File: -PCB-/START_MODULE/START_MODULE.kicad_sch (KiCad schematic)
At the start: 8 parts, among them J1 Conn_01x03_Pin, J2 Conn_01x04_Pin, U1 ATtiny85-20S, U2 TSOP382xx

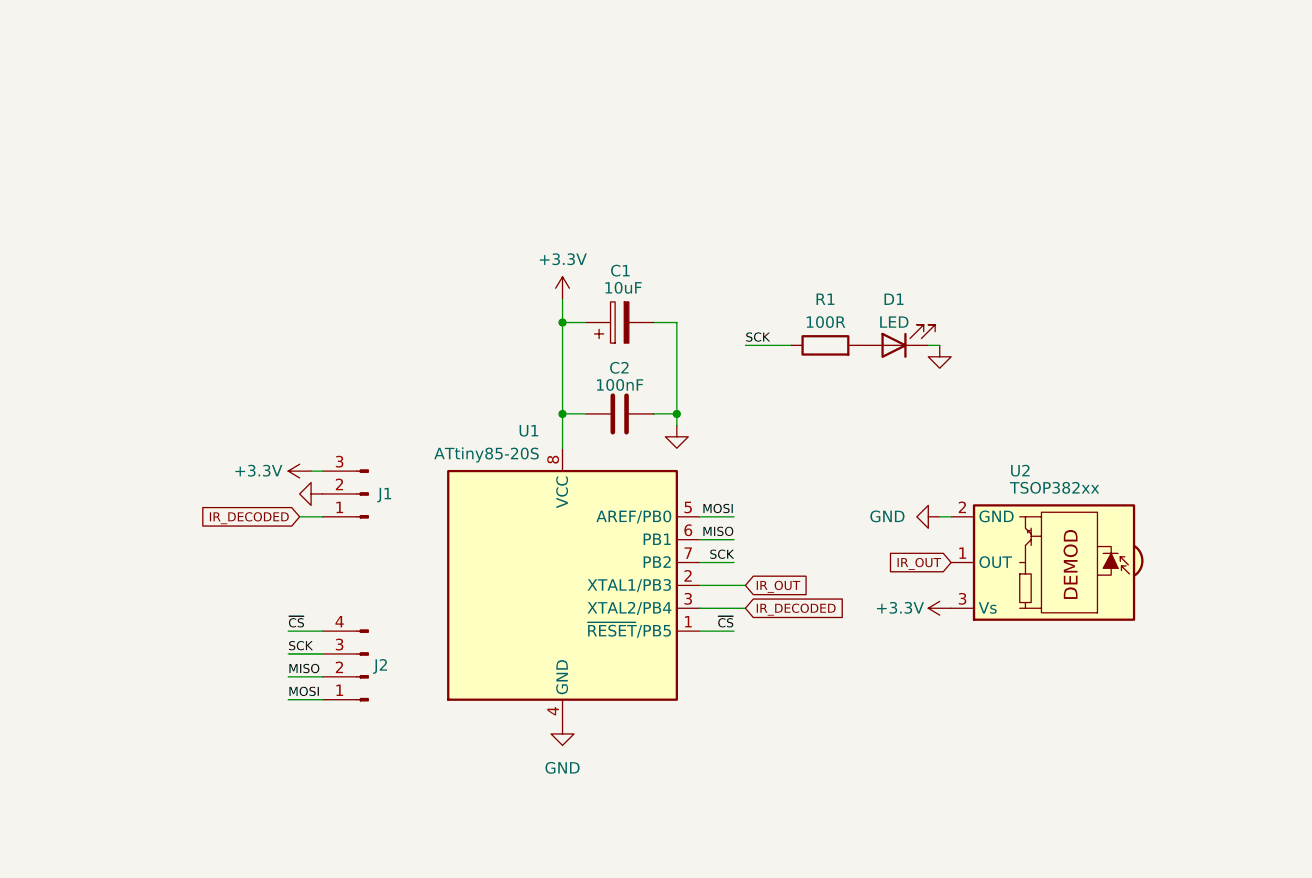
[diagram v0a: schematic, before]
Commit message: IR_module update
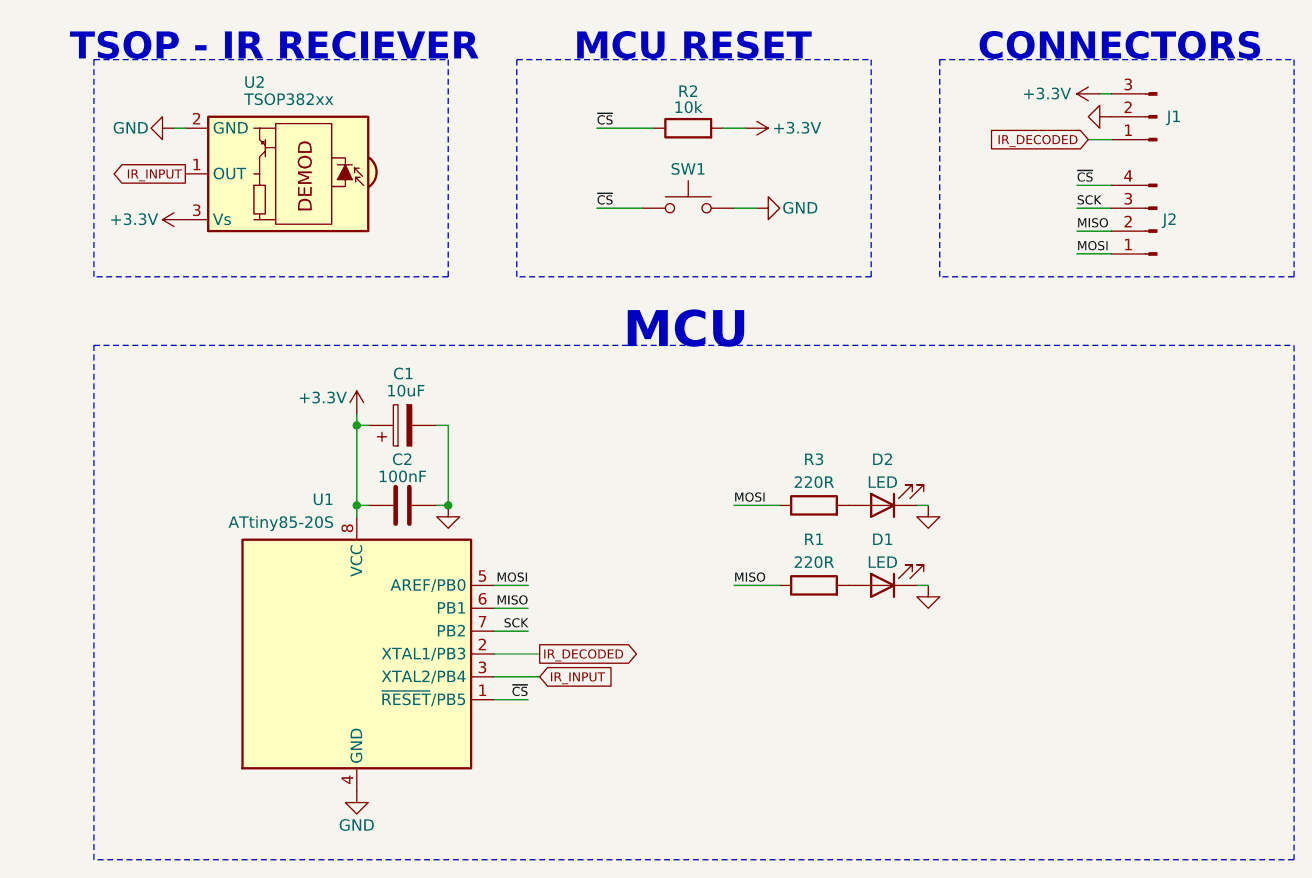
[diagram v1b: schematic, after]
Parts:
- added D2: LED, LED_SMD:LED_0805_2012Metric_Pad1.15x1.40mm_HandSolder, symbol Device:LED
- added R2: 10k, Resistor_SMD:R_0805_2012Metric_Pad1.20x1.40mm_HandSolder, symbol Device:R
- added R3: 220R, Resistor_SMD:R_0805_2012Metric_Pad1.20x1.40mm_HandSolder, symbol Device:R
- added SW1: SW_Push, sumec_brd:SW_SPST_EVQPE1, symbol Switch:SW_Push
- R1: value 100R -> 220R
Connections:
- net +3.3V: now also R2.2
- net GND: now also D2.1 (K), SW1.1
- net IR_DECODED: now also U1.2 (XTAL1/PB3); no longer U1.3 (XTAL2/PB4)
- net MISO: now also R1.1
- net MOSI: now also R3.1
- net SCK: no longer R1.1
- net ~{CS}: now also R2.1, SW1.2
- net IR_OUT renamed IR_INPUT
- net IR_INPUT: now also U1.3 (XTAL2/PB4); no longer U1.2 (XTAL1/PB3)
- new net: D2.2 (A), R3.2
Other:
- note added: "CONNECTORS"
- note added: "MCU"
- note added: "MCU RESET"
- note added: "TSOP - IR RECIEVER"
- moved on the sheet: C1, C2, D1, J1, J2, R1, U1, U2
